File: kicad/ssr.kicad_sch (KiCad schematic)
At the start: 15 parts, among them J10 ULN spare, J11 SSR S1, J12 SSR S2, J13 SSR S3, J14 SSR S4, U4 ULN2803A

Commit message: kicad: push-in spring terminals (Kangnex WJ250B), 8 A total
All 18 screw terminals replaced by Ningbo Kangnex WJ250B push-in spring
terminals (LCSC C8454 2-pole, C8420 3-pole; 3.5 mm pitch, staggered
pins, 8 A IEC). New footprints from the EasyEDA pad data and the maker
drawing (wire entry on the pin-1 side, facing the board edge) and
simple 3D models. Board total current reduced to 8 A: fuse 8 A
(Littelfuse 0154008.DR, LCSC C206919). Board: footprints swapped with
nets and schematic links kept, edges re-placed for the deeper bodies.
ERC 0; DRC unchanged (known J2/Zero-hole overlap, silk, unrouted).
Docs: BOM/README (8 A budget, 5.3 mm input path, cost ~35 EUR/board).

Co-Authored-By: Claude Opus 5.5 <noreply@anthropic.com>
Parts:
- J11, J12, J13, J14: footprint TerminalBlock_Phoenix:TerminalBlock_Phoenix_MKDS-1,5-2-5.08_1x02_P5.08mm_Horizontal -> aquaPCB:TerminalBlock_Kangnex_WJ250B-3.5-02P_P3.50mm_Staggered; LCSC (none) -> C8454; Reichelt AKL 101-02 -> (none)
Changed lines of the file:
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@@
 			)
 		)
-		(property "Footprint" "TerminalBlock_Phoenix:TerminalBlock_Phoenix_MKDS-1,5-2-5.08_1x02_P5.08mm_Horizontal"
+		(property "Footprint" "aquaPCB:TerminalBlock_Kangnex_WJ250B-3.5-02P_P3.50mm_Staggered"
 			(at 116.84 88.9 0)
 			(hide yes)
@@
 			)
 		)
-		(property "Reichelt" "AKL 101-02"
+		(property "LCSC" "C8454"
 			(at 116.84 88.9 0)
 			(hide yes)
@@
 			)
 		)
-		(property "Footprint" "TerminalBlock_Phoenix:TerminalBlock_Phoenix_MKDS-1,5-2-5.08_1x02_P5.08mm_Horizontal"
+		(property "Footprint" "aquaPCB:TerminalBlock_Kangnex_WJ250B-3.5-02P_P3.50mm_Staggered"
 			(at 116.84 109.22 0)
 			(hide yes)
@@
 			)
 		)
-		(property "Reichelt" "AKL 101-02"
+		(property "LCSC" "C8454"
 			(at 116.84 109.22 0)
 			(hide yes)
@@
 			)
 		)
-		(property "Footprint" "TerminalBlock_Phoenix:TerminalBlock_Phoenix_MKDS-1,5-2-5.08_1x02_P5.08mm_Horizontal"
+		(property "Footprint" "aquaPCB:TerminalBlock_Kangnex_WJ250B-3.5-02P_P3.50mm_Staggered"
 			(at 116.84 119.38 0)
 			(hide yes)
@@
 			)
 		)
-		(property "Reichelt" "AKL 101-02"
+		(property "LCSC" "C8454"
 			(at 116.84 119.38 0)
 			(hide yes)
@@
 			)
 		)
-		(property "Footprint" "TerminalBlock_Phoenix:TerminalBlock_Phoenix_MKDS-1,5-2-5.08_1x02_P5.08mm_Horizontal"
+		(property "Footprint" "aquaPCB:TerminalBlock_Kangnex_WJ250B-3.5-02P_P3.50mm_Staggered"
 			(at 116.84 99.06 0)
 			(hide yes)
@@
 			)
 		)
-		(property "Reichelt" "AKL 101-02"
+		(property "LCSC" "C8454"
 			(at 116.84 99.06 0)
 			(hide yes)

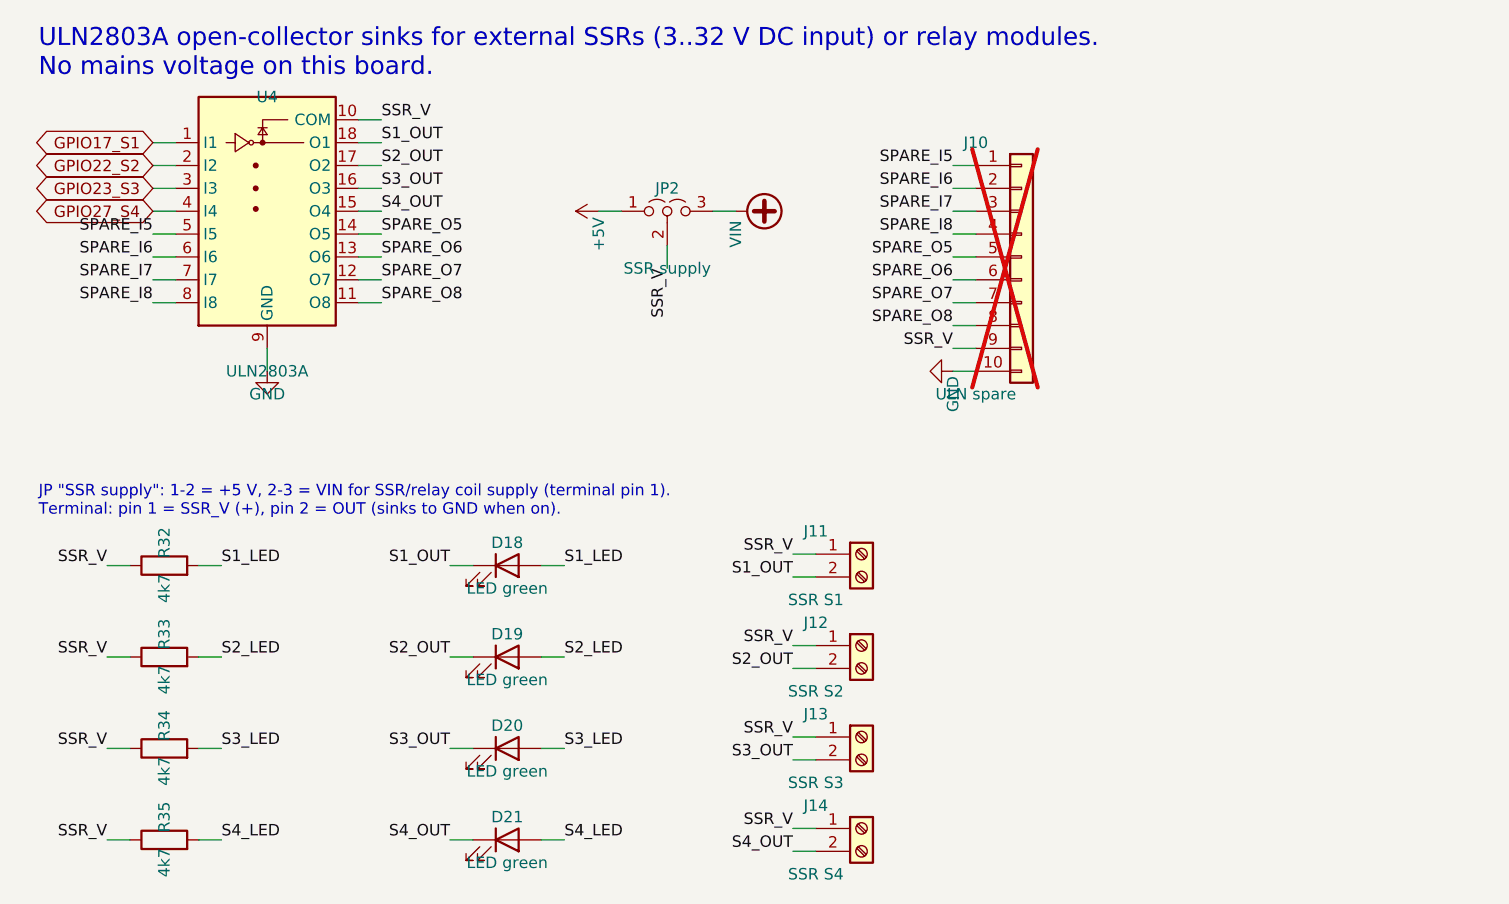
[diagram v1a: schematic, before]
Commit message: kicad: routing progress (by hand)
Co-Authored-By: Claude Opus 5.5 (1M context) <noreply@anthropic.com>
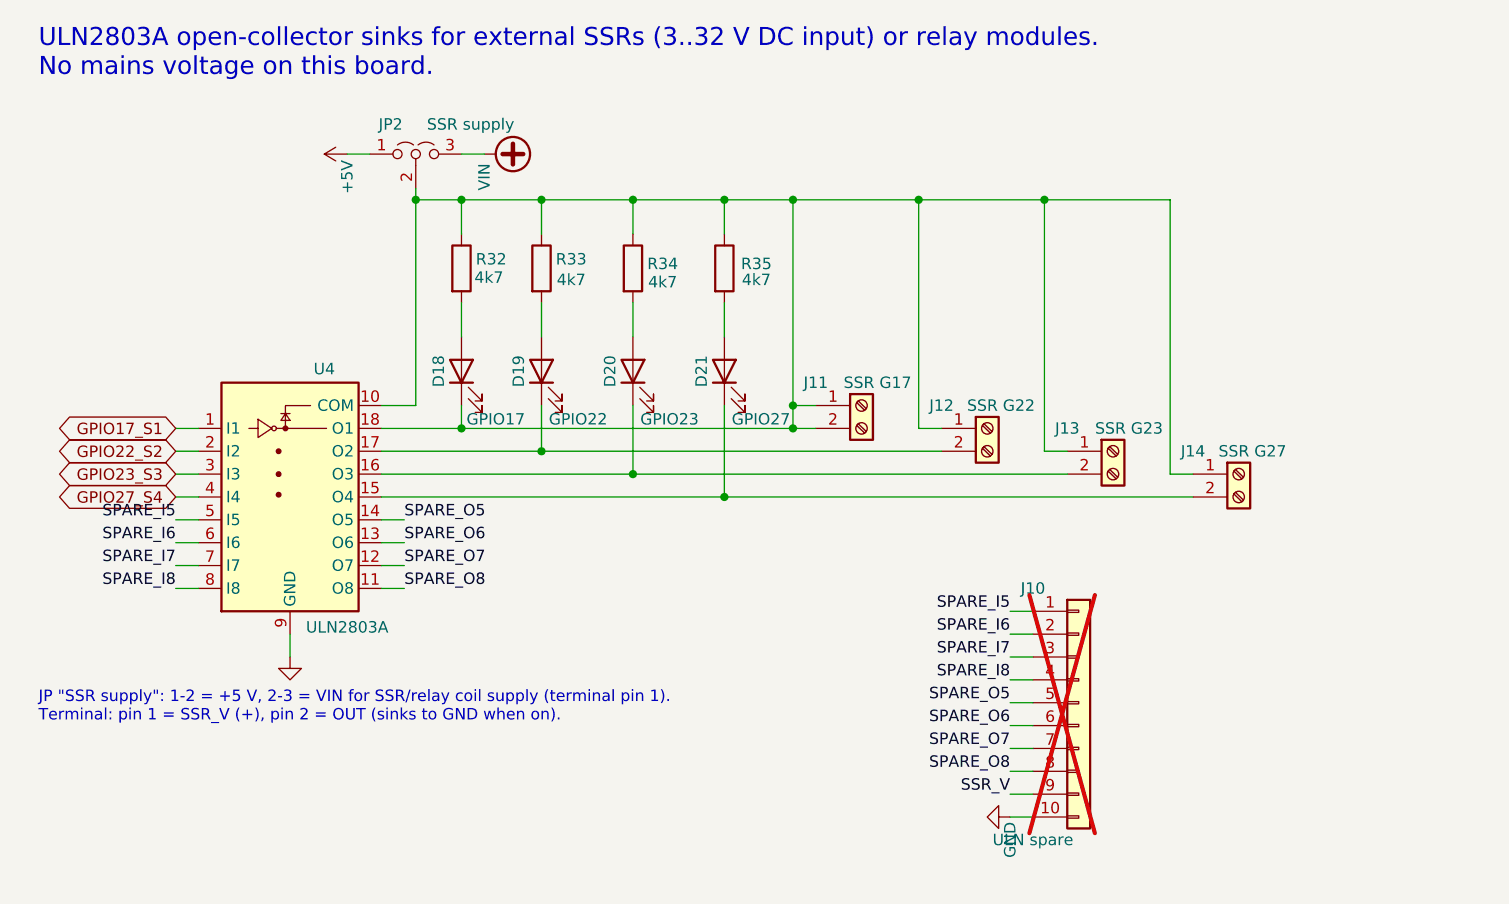
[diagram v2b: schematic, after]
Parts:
- D18: value LED green -> GPIO17
- D19: value LED green -> GPIO22
- D20: value LED green -> GPIO23
- D21: value LED green -> GPIO27
- J11: value SSR S1 -> SSR G17
- J12: value SSR S2 -> SSR G22
- J13: value SSR S3 -> SSR G23
- J14: value SSR S4 -> SSR G27
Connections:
- net SSR_V: no longer J11.1 (Pin_1), J12.1 (Pin_1), J13.1 (Pin_1), J14.1 (Pin_1), JP2.2 (C), R32.1, R33.1, R34.1, R35.1, U4.10 (COM)
- net S1_LED: no longer names the net of D18.2 (A), R32.2
- net S1_OUT: no longer names the net of D18.1 (K), J11.2 (Pin_2), U4.18 (O1)
- net S1_OUT: now also J11.1 (Pin_1), J12.1 (Pin_1), J13.1 (Pin_1), J14.1 (Pin_1), JP2.2 (C), R32.1, R33.1, R34.1, R35.1, U4.10 (COM)
- net S2_LED: no longer names the net of D19.2 (A), R33.2
- net S2_OUT: no longer names the net of D19.1 (K), J12.2 (Pin_2), U4.17 (O2)
- net S3_LED: no longer names the net of D20.2 (A), R34.2
- net S3_OUT: no longer names the net of D20.1 (K), J13.2 (Pin_2), U4.16 (O3)
- net S4_LED: no longer names the net of D21.2 (A), R35.2
- net S4_OUT: no longer names the net of D21.1 (K), J14.2 (Pin_2), U4.15 (O4)
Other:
- moved on the sheet: D18, D19, D20, D21, J10, J11, J12, J13, J14, JP2, R32, R33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
